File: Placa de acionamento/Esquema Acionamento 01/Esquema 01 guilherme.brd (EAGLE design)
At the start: 66 x 57.2 mm, 22 parts, among them Q1 IRF540, Q2 IRF540, Q3 IRF540

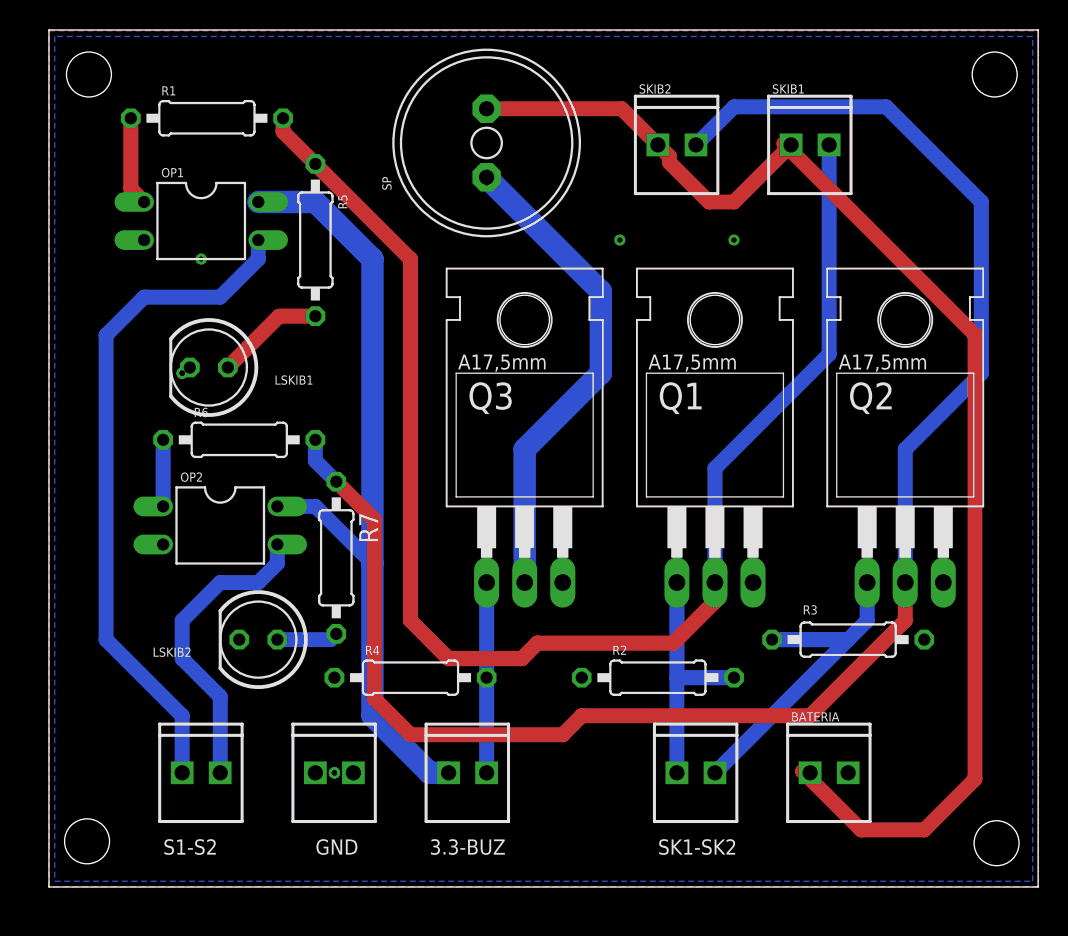
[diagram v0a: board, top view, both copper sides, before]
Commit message: Add files via upload
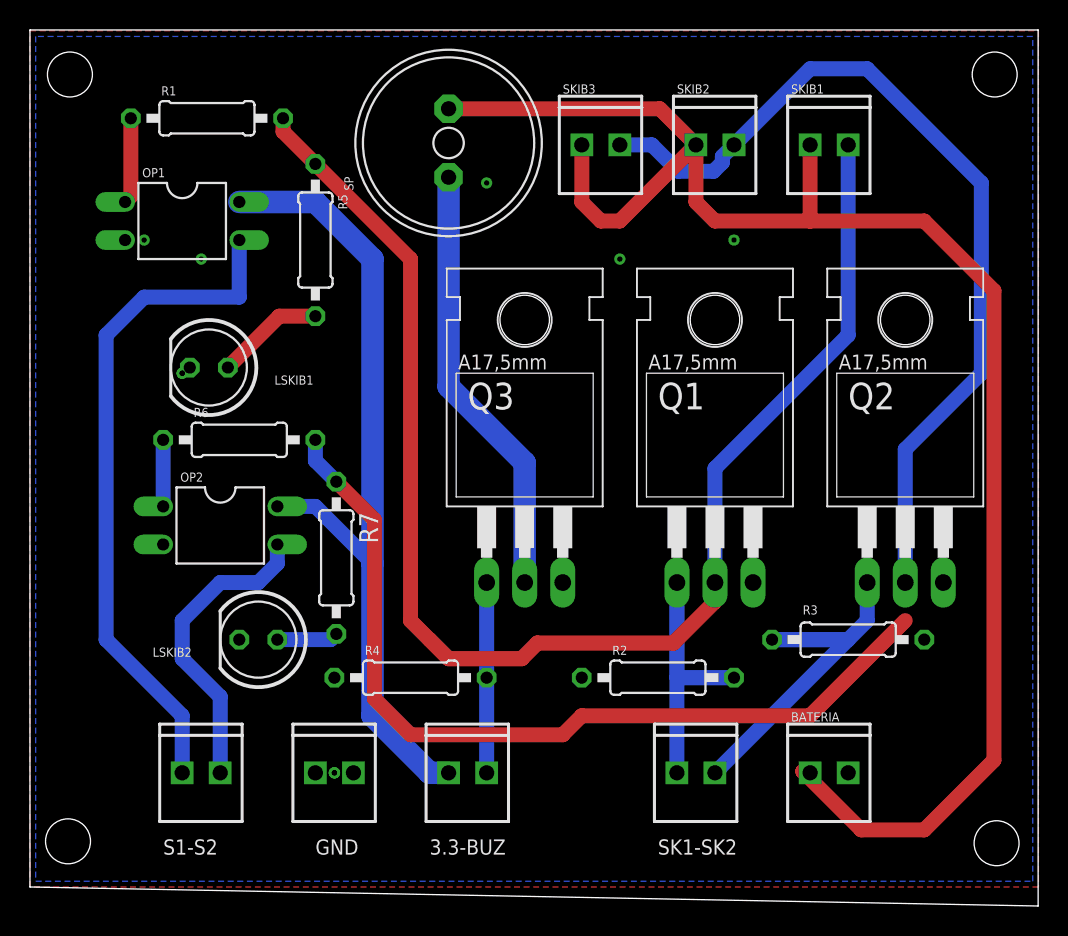
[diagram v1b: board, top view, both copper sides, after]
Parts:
- added SKIB3: (no value), SparkFun-Connectors:1X02_2.54_SCREWTERM
- moved SKIB2 2.54 mm to (43.2, 49.5)
- moved SP 2.54 mm to (26.7, 49.7)
- moved OP1 1.27 mm to (8.89, 44.5)
- moved SKIB1 1.27 mm to (50.8, 49.5)
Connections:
- net SKIB2_CONECTOR: now also SKIB3.P1
- net VCC: now also SKIB3.P2
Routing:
- net VCC: track 87.5 -> 111.0 mm
- net SKIB2_CONECTOR: track 111.3 -> 118.3 mm
- net N$2: track 32.3 -> 29.2 mm
- net 3.3V: track 54.3 -> 55.5 mm
- net SKIB1_CONECTOR: track 93.6 -> 94.2 mm
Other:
- board size 66 x 57.2 mm -> 67.3 x 58.5 mm
